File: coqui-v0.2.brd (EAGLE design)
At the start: 75.8 x 18 mm, 33 parts, among them IC3 MCP73831, IC4 MCP1700-33, J1 AYZ0202

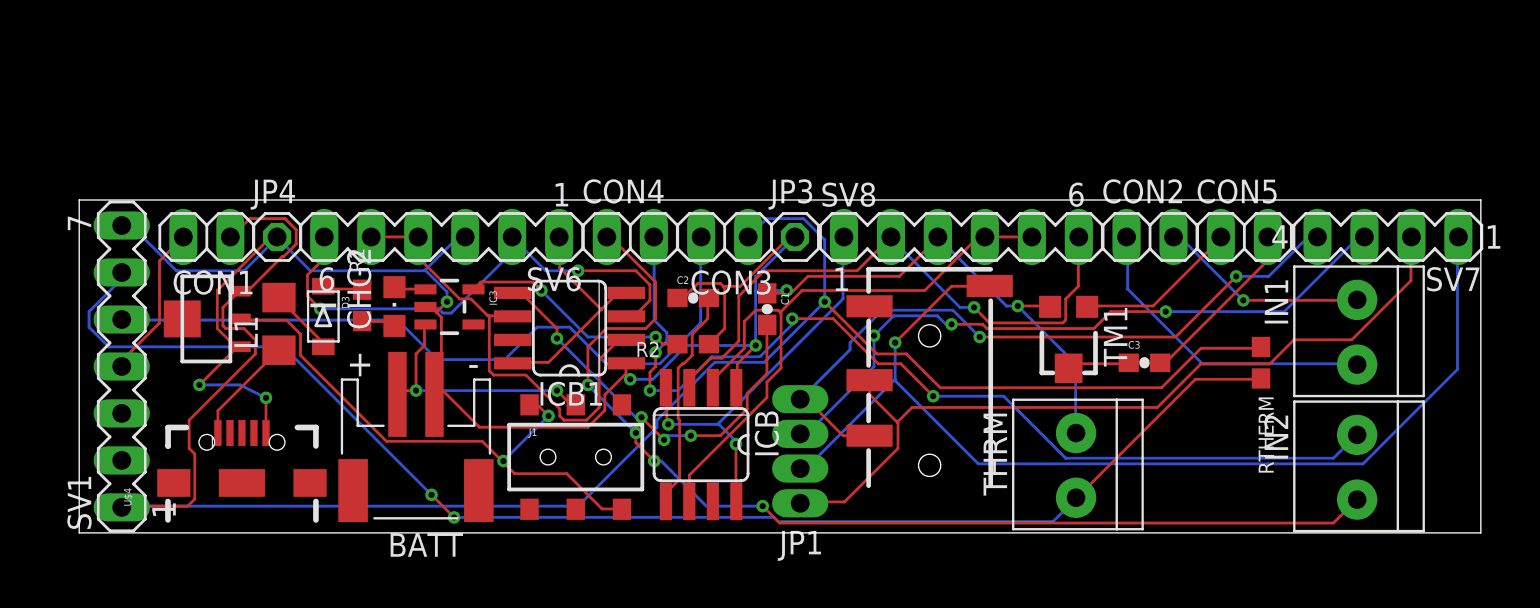
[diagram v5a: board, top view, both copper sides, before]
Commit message: update
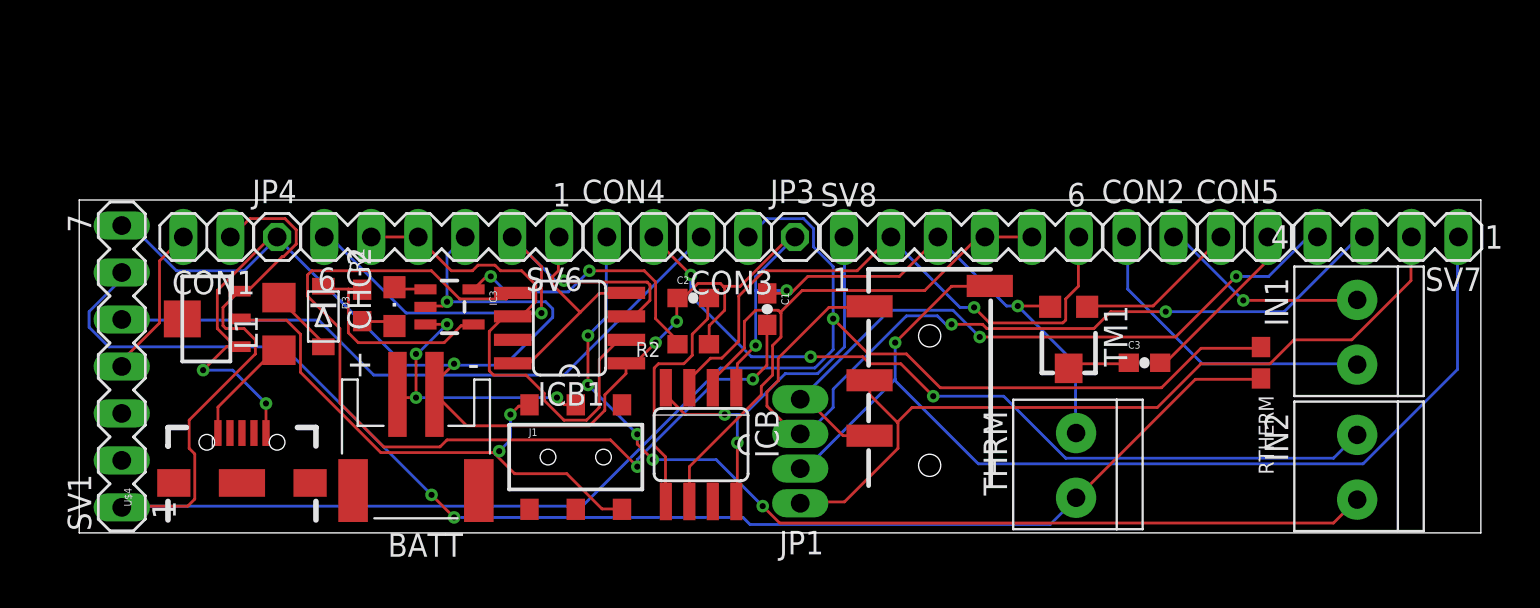
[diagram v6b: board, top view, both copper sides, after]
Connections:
- removed net VIN: IC3.4
- net VBUS: now also IC3.4
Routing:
- net N$2: track 22.0 -> 49.1 mm, vias 4 -> 2
- net VBUS: track 2.17 -> 11.9 mm
- net N$8: track 38.2 -> 47.4 mm, vias 3 -> 2
- net GND: track 117.6 -> 126.3 mm, vias 7 -> 9
- net N$16: track 52.6 -> 44.2 mm, vias 4 -> 3
- net N$19: track 39.3 -> 35.7 mm
- net N$17: track 57.5 -> 53.9 mm, vias 4 -> 5
- net N$1: track 25.1 -> 28.5 mm
- net N$3: track 12.6 -> 15.1 mm
- net VBAT: track 13.8 -> 15.7 mm, vias 2 -> 4
- net N$14: track 12.1 -> 13.3 mm
- net VCC: track 105.4 -> 106.6 mm
- net AOUT1: track 28.5 -> 29.2 mm
